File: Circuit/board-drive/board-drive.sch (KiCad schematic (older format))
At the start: 29 parts, among them P1 XT30, P10 XT60, P2 XT30, P3 XT30, P4 XT30, P5 XT30, P6 XT30, P7 XT30, P8 XT30, P9 XT60, U1 Pololu_Maestro12, U10 PowerDist_WiretoBoard, U11 PowerDist_WiretoBoard, U16 PowerDist_WiretoBoard, U17 PowerDist_WiretoBoard, U18 PowerDist_WiretoBoard, U19 PowerDist_WiretoBoard, U2 Si8660BA-B-IS1, U3 Si8660BA-B-IS1, U8 PowerDist_WiretoBoard, U9 PowerDist_WiretoBoard

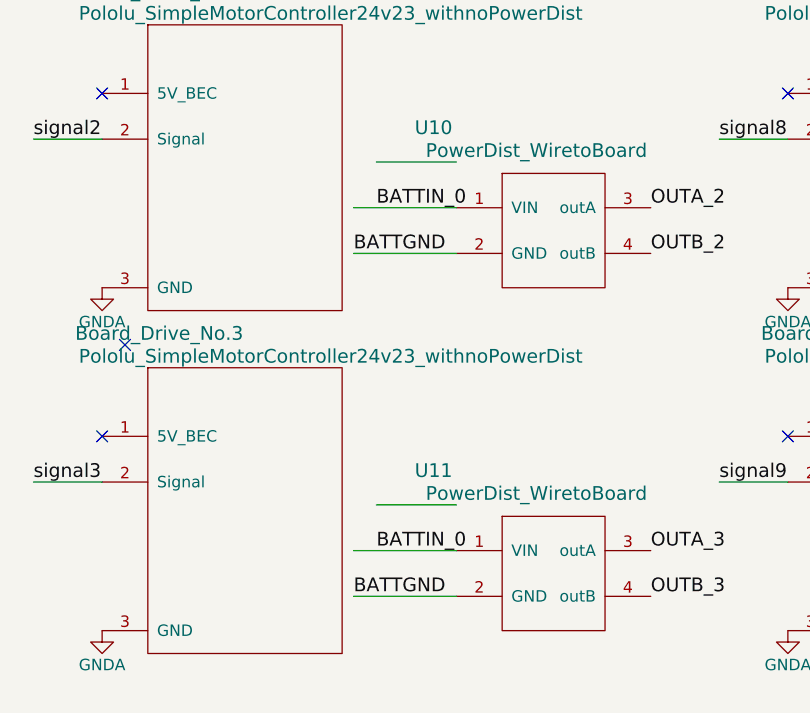
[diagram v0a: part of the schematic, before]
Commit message: edited pcb
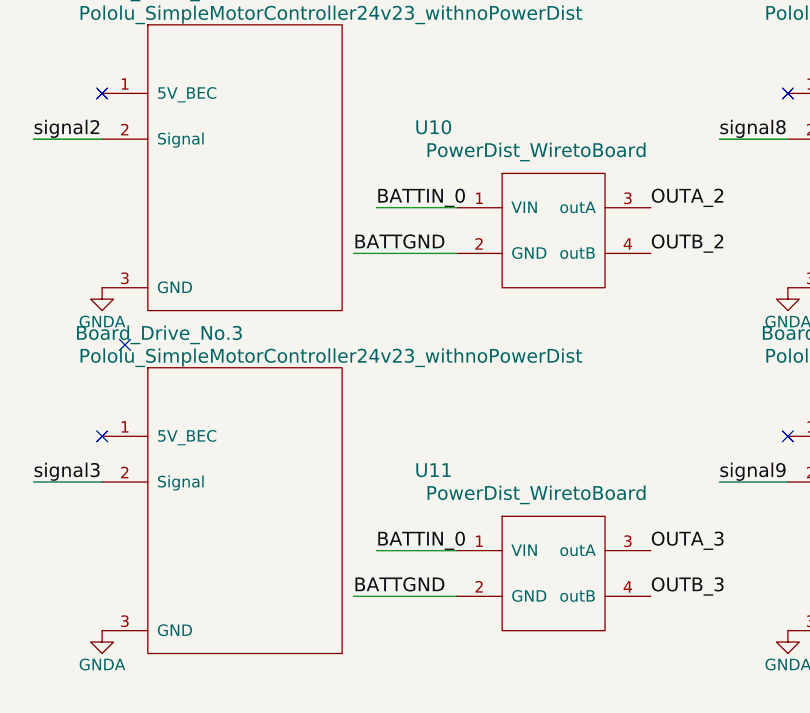
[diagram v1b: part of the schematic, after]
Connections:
- wire segments 87 -> 85
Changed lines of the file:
@@
 LIBS:contrib
 LIBS:valves
+LIBS:zeabus
 LIBS:board-drive-cache
 EELAYER 25 0
@@
 	6800 3150 6350 3150
 Wire Wire Line
-	6450 4300 6800 4300
-Wire Wire Line
-	6800 4500 6350 4500
-Wire Wire Line
-	6450 5800 6800 5800
-Wire Wire Line
-	6800 6000 6350 6000
-Wire Wire Line
 	9350 6200 9800 6200
 Wire Wire Line
@@
 	7900 2500 8250 2500
 NoConn ~ 5250 2500
+Wire Wire Line
+	6450 4500 6800 4500
+Wire Wire Line
+	6450 6000 6800 6000
 $EndSCHEMATC
